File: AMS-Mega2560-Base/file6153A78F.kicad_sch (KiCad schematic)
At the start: 11 parts, among them Q1 2N7000, Q2 2N7000, Q3 2N7000

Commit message: fixing some library settings and updating some schematics
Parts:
- R10, R11, R12, R5, R6, R7, R8, R9: footprint Resistor_THT:R_Axial_DIN0207_L6.3mm_D2.5mm_P5.08mm_Vertical -> Resistor_THT:R_Axial_DIN0207_L6.3mm_D2.5mm_P2.54mm_Vertical
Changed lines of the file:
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@@
       (effects (font (size 1.27 1.27)) (justify left))
     )
-    (property "Footprint" "Resistor_THT:R_Axial_DIN0207_L6.3mm_D2.5mm_P5.08mm_Vertical" (id 2) (at 107.442 138.43 90)
+    (property "Footprint" "Resistor_THT:R_Axial_DIN0207_L6.3mm_D2.5mm_P2.54mm_Vertical" (id 2) (at 107.442 138.43 90)
       (effects (font (size 1.27 1.27)) hide)
     )
@@
       (effects (font (size 1.27 1.27)) (justify left))
     )
-    (property "Footprint" "Resistor_THT:R_Axial_DIN0207_L6.3mm_D2.5mm_P5.08mm_Vertical" (id 2) (at 181.102 64.77 90)
+    (property "Footprint" "Resistor_THT:R_Axial_DIN0207_L6.3mm_D2.5mm_P2.54mm_Vertical" (id 2) (at 181.102 64.77 90)
       (effects (font (size 1.27 1.27)) hide)
     )
@@
       (effects (font (size 1.27 1.27)) (justify left))
     )
-    (property "Footprint" "Resistor_THT:R_Axial_DIN0207_L6.3mm_D2.5mm_P5.08mm_Vertical" (id 2) (at 106.172 99.06 90)
+    (property "Footprint" "Resistor_THT:R_Axial_DIN0207_L6.3mm_D2.5mm_P2.54mm_Vertical" (id 2) (at 106.172 99.06 90)
       (effects (font (size 1.27 1.27)) hide)
     )
@@
       (effects (font (size 1.27 1.27)) (justify left))
     )
-    (property "Footprint" "Resistor_THT:R_Axial_DIN0207_L6.3mm_D2.5mm_P5.08mm_Vertical" (id 2) (at 145.542 100.33 90)
+    (property "Footprint" "Resistor_THT:R_Axial_DIN0207_L6.3mm_D2.5mm_P2.54mm_Vertical" (id 2) (at 145.542 100.33 90)
       (effects (font (size 1.27 1.27)) hide)
     )
@@
       (effects (font (size 1.27 1.27)) (justify left))
     )
-    (property "Footprint" "Resistor_THT:R_Axial_DIN0207_L6.3mm_D2.5mm_P5.08mm_Vertical" (id 2) (at 137.922 100.33 90)
+    (property "Footprint" "Resistor_THT:R_Axial_DIN0207_L6.3mm_D2.5mm_P2.54mm_Vertical" (id 2) (at 137.922 100.33 90)
       (effects (font (size 1.27 1.27)) hide)
     )
@@
       (effects (font (size 1.27 1.27)) (justify left))
     )
-    (property "Footprint" "Resistor_THT:R_Axial_DIN0207_L6.3mm_D2.5mm_P5.08mm_Vertical" (id 2) (at 106.172 57.15 90)
+    (property "Footprint" "Resistor_THT:R_Axial_DIN0207_L6.3mm_D2.5mm_P2.54mm_Vertical" (id 2) (at 106.172 57.15 90)
       (effects (font (size 1.27 1.27)) hide)
     )
@@
       (effects (font (size 1.27 1.27)) (justify left))
     )
-    (property "Footprint" "Resistor_THT:R_Axial_DIN0207_L6.3mm_D2.5mm_P5.08mm_Vertical" (id 2) (at 145.542 58.42 90)
+    (property "Footprint" "Resistor_THT:R_Axial_DIN0207_L6.3mm_D2.5mm_P2.54mm_Vertical" (id 2) (at 145.542 58.42 90)
       (effects (font (size 1.27 1.27)) hide)
     )
@@
       (effects (font (size 1.27 1.27)) (justify left))
     )
-    (property "Footprint" "Resistor_THT:R_Axial_DIN0207_L6.3mm_D2.5mm_P5.08mm_Vertical" (id 2) (at 137.922 58.42 90)
-      (effects (font (size 1.27 1.27)) hide)
-    )
+    (property "Footprint" "Resistor_THT:R_Axial_DIN0207_L6.3mm_D2.5mm_P2.54mm_Vertical" (id 2) (at 137.922 58.42 90)
+      (effects (font (size 1.27 1.27)) hide)
+    )

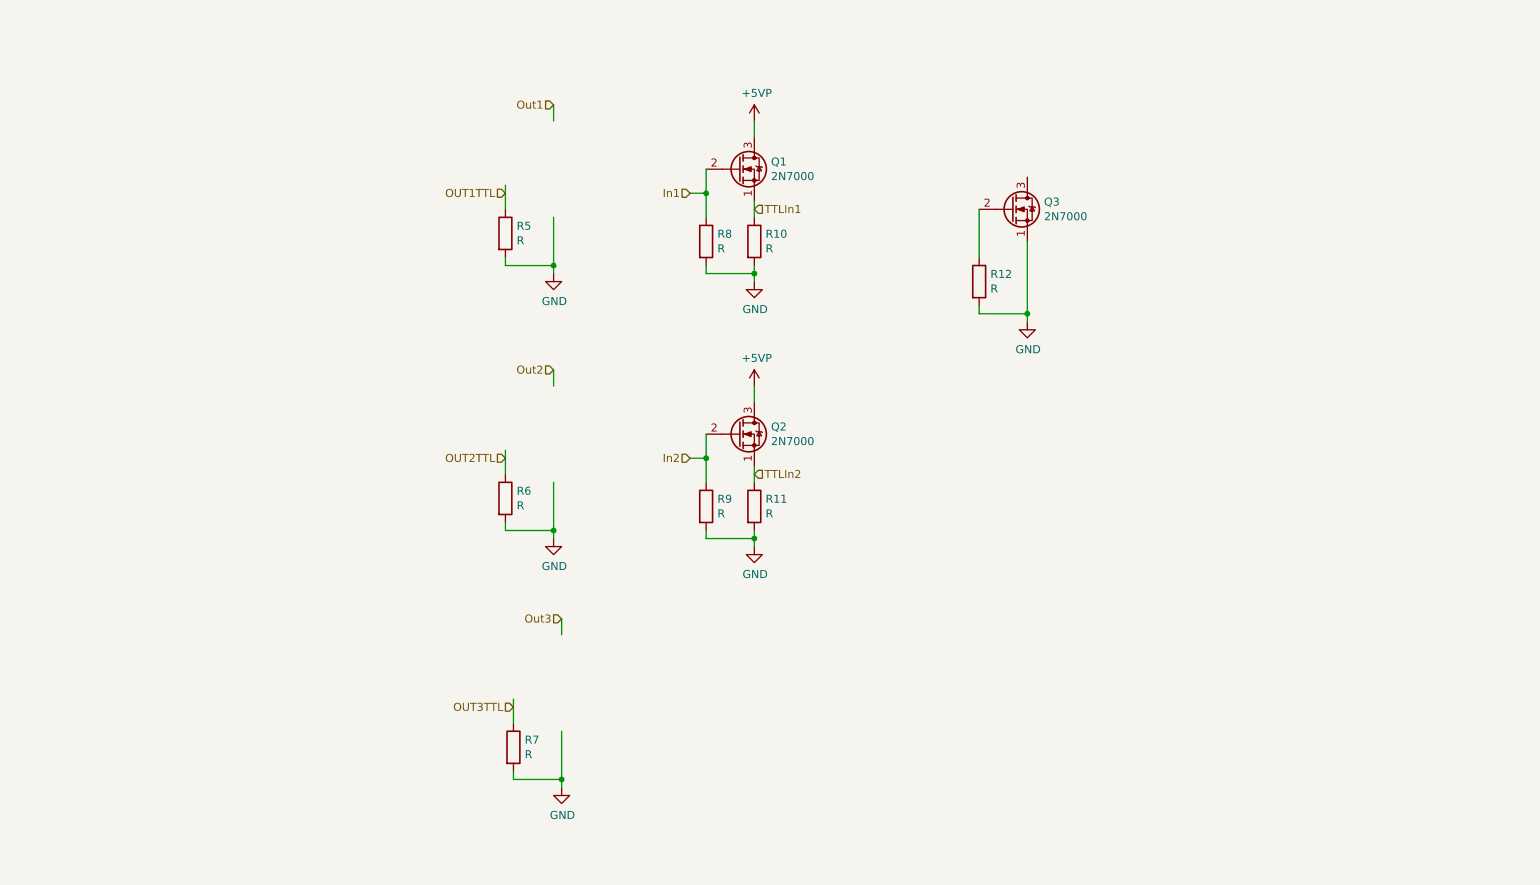
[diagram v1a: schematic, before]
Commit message: BaseBoard fixes and updates. doing schematic work.
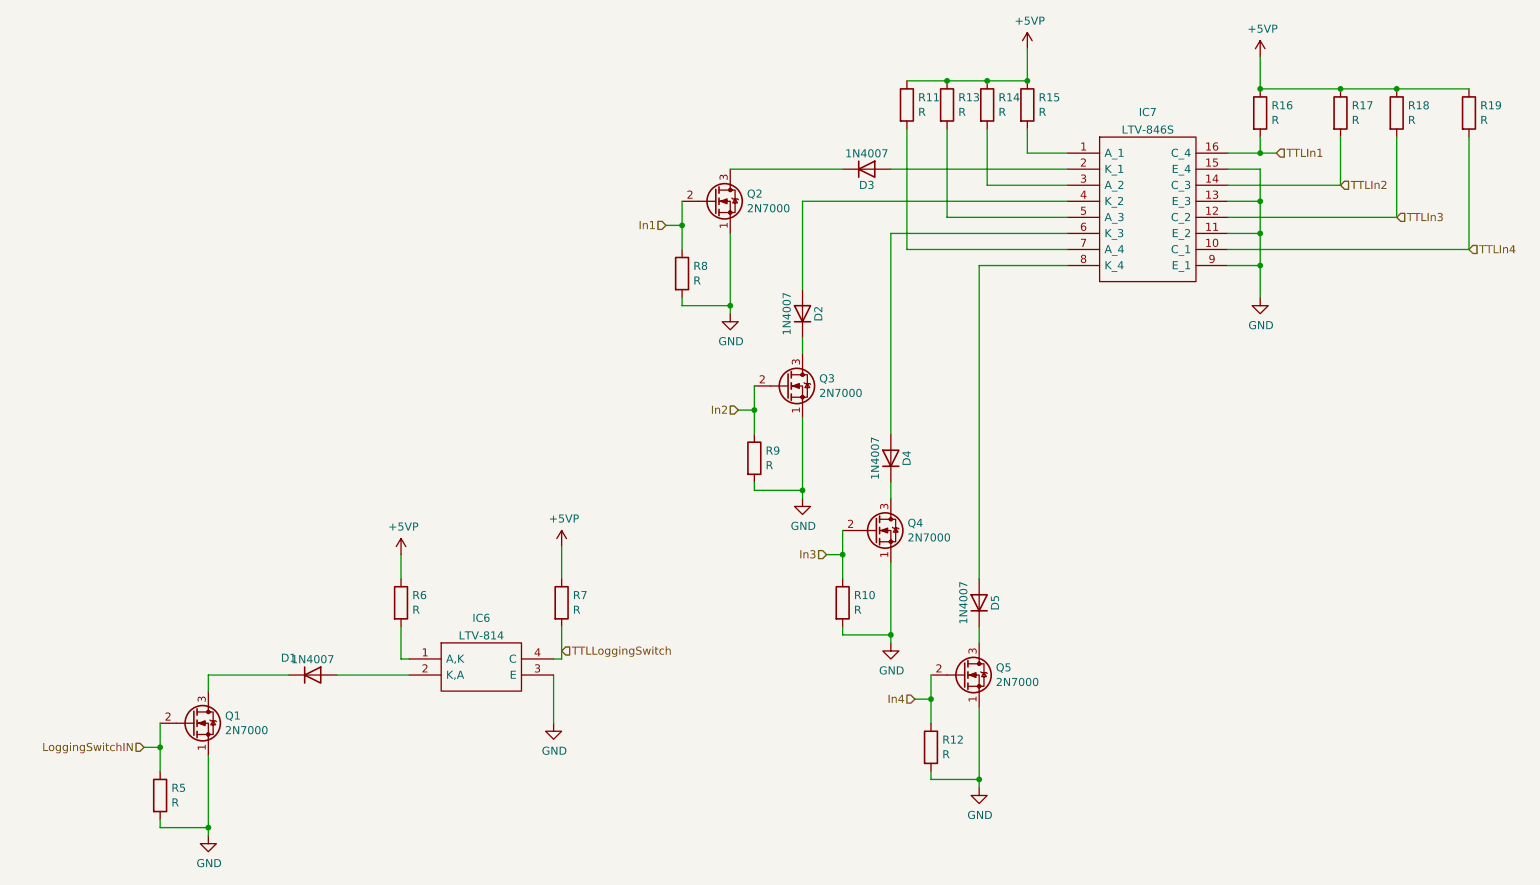
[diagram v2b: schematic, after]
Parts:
- removed Q3: 2N7000, Package_TO_SOT_THT:TO-92_Inline, symbol Transistor_FET:2N7000
- added D1, D2, D3, D4, D5: 1N4007, Diode_THT:D_DO-41_SOD81_P10.16mm_Horizontal, symbol Diode:1N4007
- added IC6: LTV-814, SamacSys_Parts:DIP762W60P254L460H450Q4N, symbol Samac_Sys:LTV-814
- added IC7: LTV-846S, SOP254P1016X460-16N, symbol Samac_Sys:LTV-846S
- added Q1, Q4, Q5: 2N7000, Package_TO_SOT_THT:TO-92_Inline, symbol Transistor_FET:2N7000
- added R10, R11, R13, R14, R16, R18, R19: R, Resistor_THT:R_Axial_DIN0207_L6.3mm_D2.5mm_P2.54mm_Vertical, symbol Device:R
- renumbered Q1 to Q2, Q2 to Q3, R10 to R15, R11 to R17
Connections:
- net OUT2TTL is gone; now on net +5VP: R6.1
- net OUT3TTL is gone; now on net +5VP: R7.1
- net +5VP: now also R15.1, R17.1, R11.1, R13.1, R14.1, R16.1, R18.1, R19.1; no longer Q2.3 (D), Q3.3 (D)
- net GND: now also Q2.1 (S), Q3.1 (S), IC6.3 (E), IC7.11 (E_2), IC7.13 (E_3), IC7.15 (E_4), IC7.9 (E_1), Q1.1 (S), Q4.1 (S), Q5.1 (S), R10.2; no longer R15.2, R17.2, R6.2, R7.2
- net TTLIn1: now also IC7.16 (C_4), R16.2; no longer Q2.1 (S), R15.1
- net TTLIn2: now also R17.2, IC7.14 (C_3); no longer Q3.1 (S), R17.1
- net In4: now reaches R12.1
- net In4: now also Q5.2 (G)
- net OUT1TTL renamed LoggingSwitchIN
- net LoggingSwitchIN: now also Q1.2 (G)
- new net: D2.1 (K), Q3.3 (D)
- new net: D3.1 (K), Q2.3 (D)
- new net: IC7.1 (A_1), R15.2
- new net: IC7.3 (A_2), R14.2
- new net: IC7.5 (A_3), R13.2
- new net: D3.2 (A), IC7.2 (K_1)
- new net: D5.1 (K), Q5.3 (D)
- new net: D5.2 (A), IC7.8 (K_4)
- new net: IC6.1 (A,K), R6.2
- new net: D2.2 (A), IC7.4 (K_2)
- new net: IC7.7 (A_4), R11.2
- new net: D1.2 (A), IC6.2 (K,A)
- new net: D1.1 (K), Q1.3 (D)
- new net: D4.1 (K), Q4.3 (D)
- new net: D4.2 (A), IC7.6 (K_3)
- new net In3: Q4.2 (G), R10.1
- new net TTLIn3: IC7.12 (C_2), R18.2
- new net TTLIn4: IC7.10 (C_1), R19.2
- new net TTLLoggingSwitch: IC6.4 (C), R7.2
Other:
- moved on the sheet: Q2, Q3, R15, R17, R8, R9
